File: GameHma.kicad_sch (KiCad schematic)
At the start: 15 parts, among them J1 Screw_Terminal_01x02, J2 Motor_Terminal_01x04, J3 Motor_Terminal_01x04, J4 Motor_Terminal_01x04, J5 Motor_Terminal_01x04, U1 ESP32-DEVKIT-V1, U2 A4988_STEPPER_MOTOR_DRIVER_CA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, U3 A4988_STEPPER_MOTOR_DRIVER_CA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, U4 A4988_STEPPER_MOTOR_DRIVER_CA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, U5 A4988_STEPPER_MOTOR_DRIVER_CA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, U6 SRT_MP1584EN

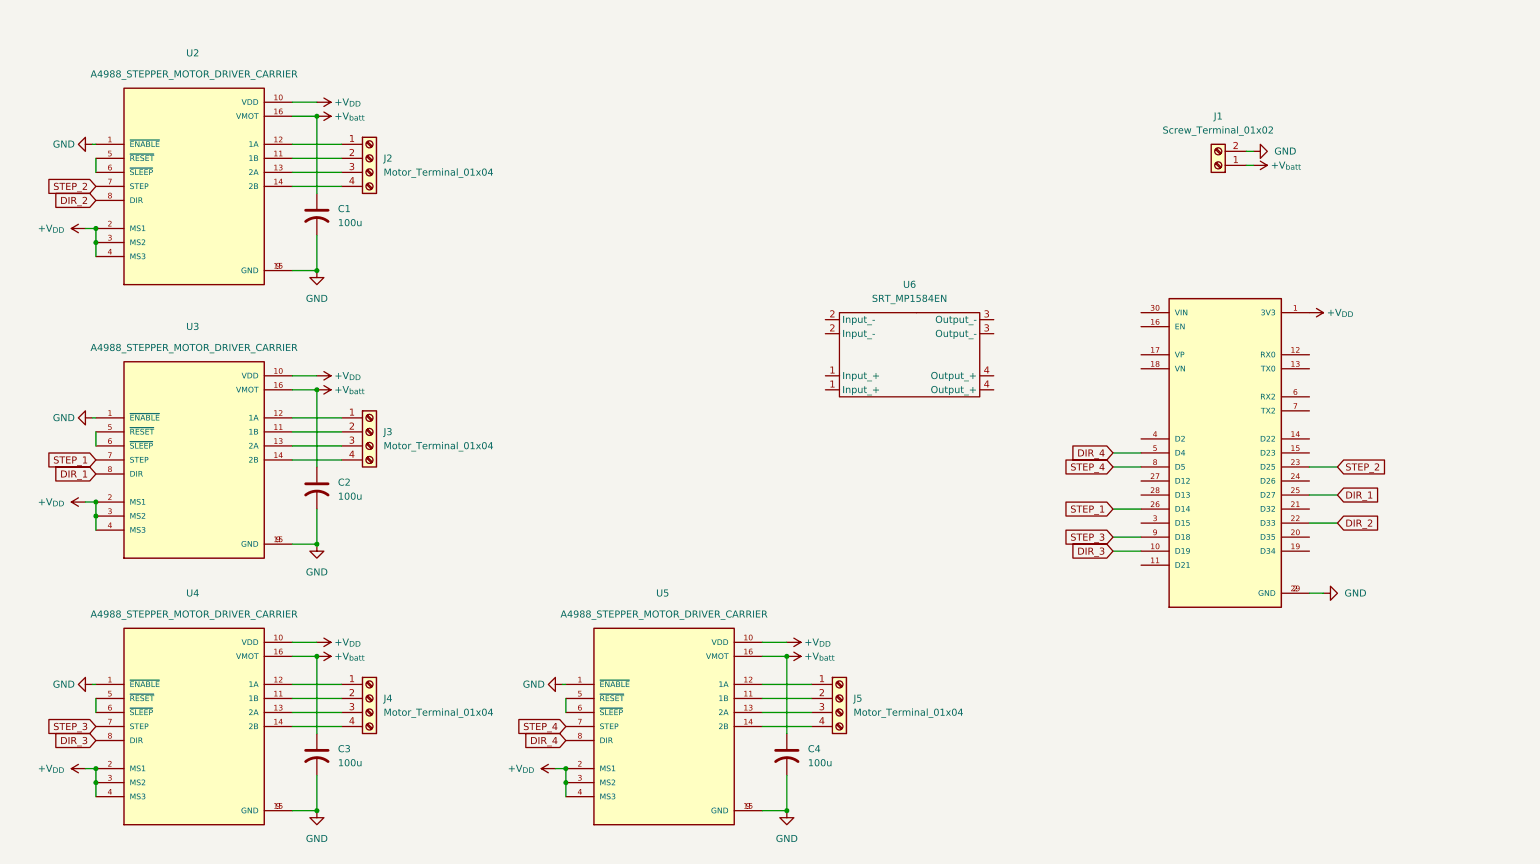
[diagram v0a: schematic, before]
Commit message: Organize and add names
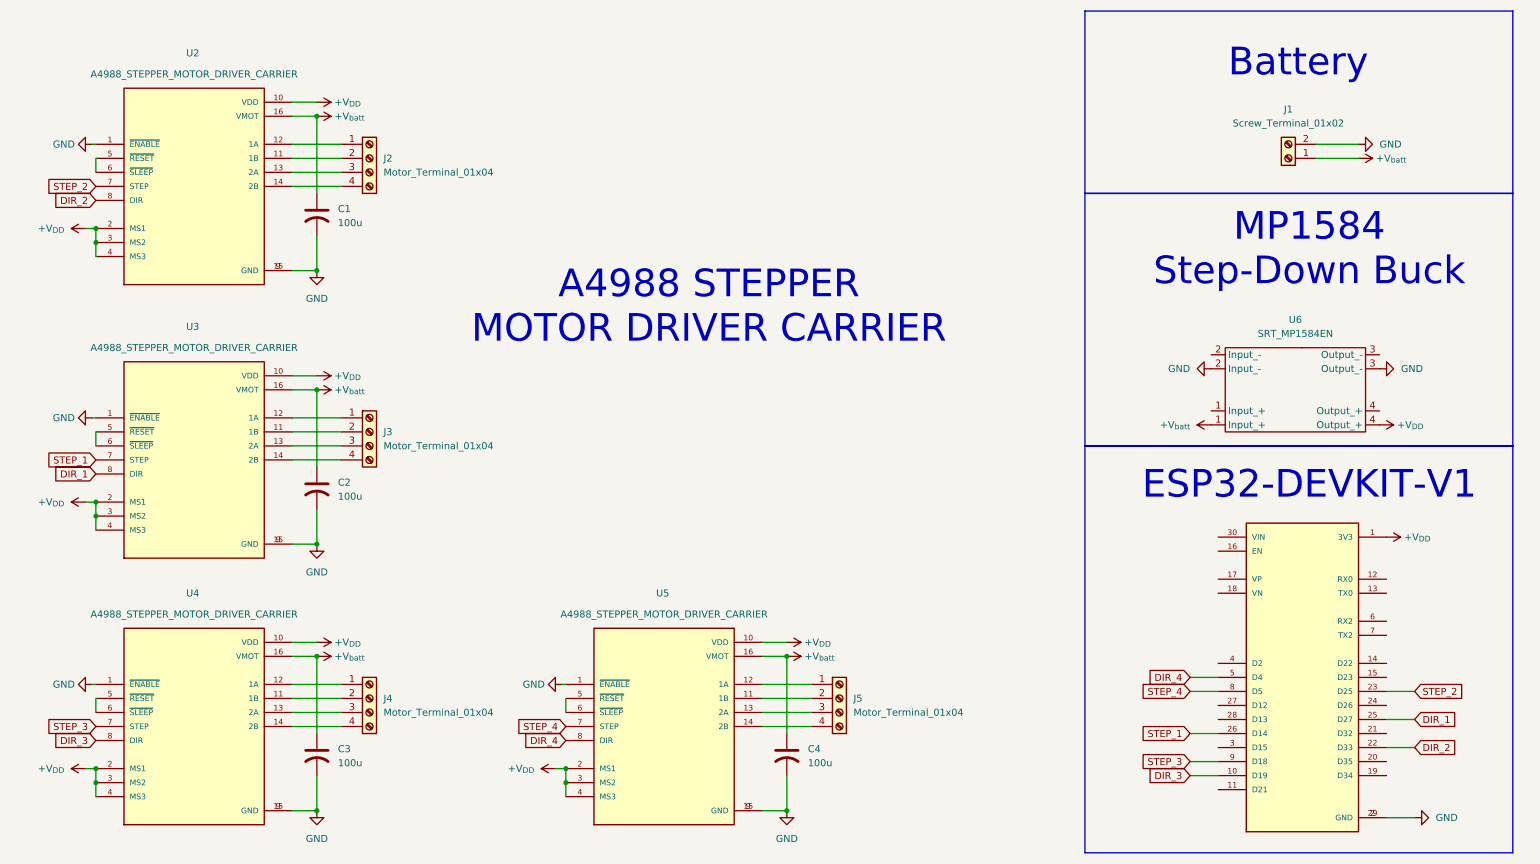
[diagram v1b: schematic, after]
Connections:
- net +V_{DD}: now also U6.4 (Output_+)
- net +V_{batt}: now also U6.1 (Input_+)
- net GND: now also U6.2 (Input_-), U6.3 (Output_-)
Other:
- note added: "A4988 STEPPER MOTOR DRIVER CARRIER"
- note added: "Battery"
- note added: "ESP32-DEVKIT-V1"
- note added: "MP1584 Step-Down Buck"
- moved on the sheet: J1, U6
